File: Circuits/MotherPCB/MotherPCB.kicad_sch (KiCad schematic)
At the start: 1 part, among them U20 Teensy_4.1

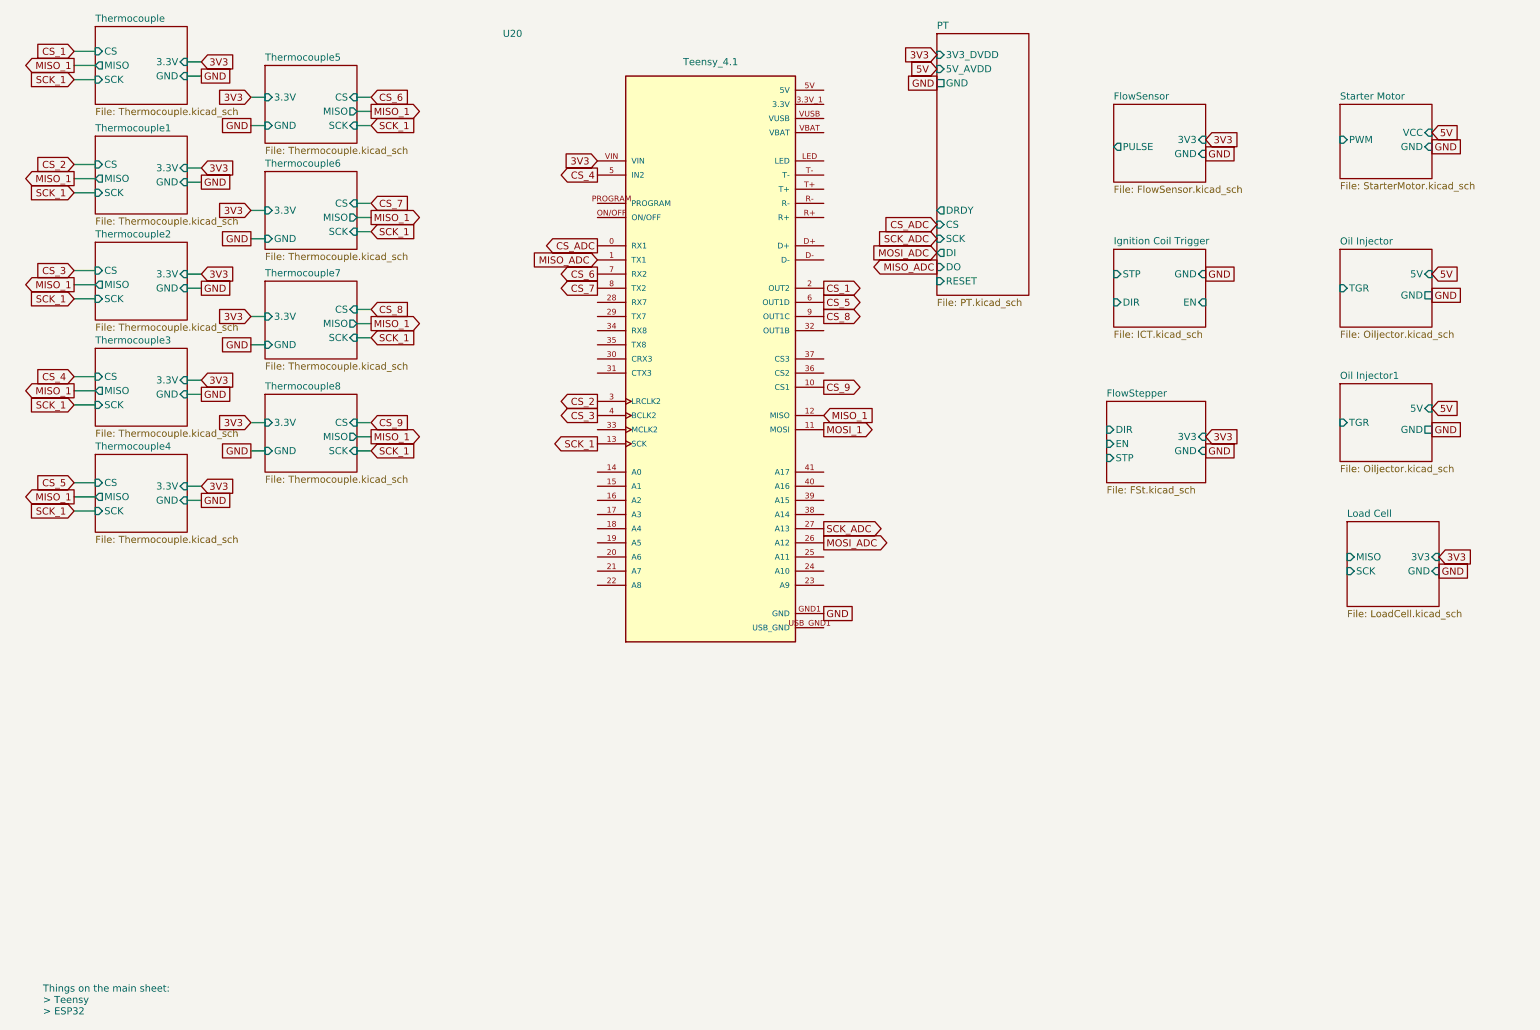
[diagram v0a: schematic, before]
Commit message: Schematic Finished
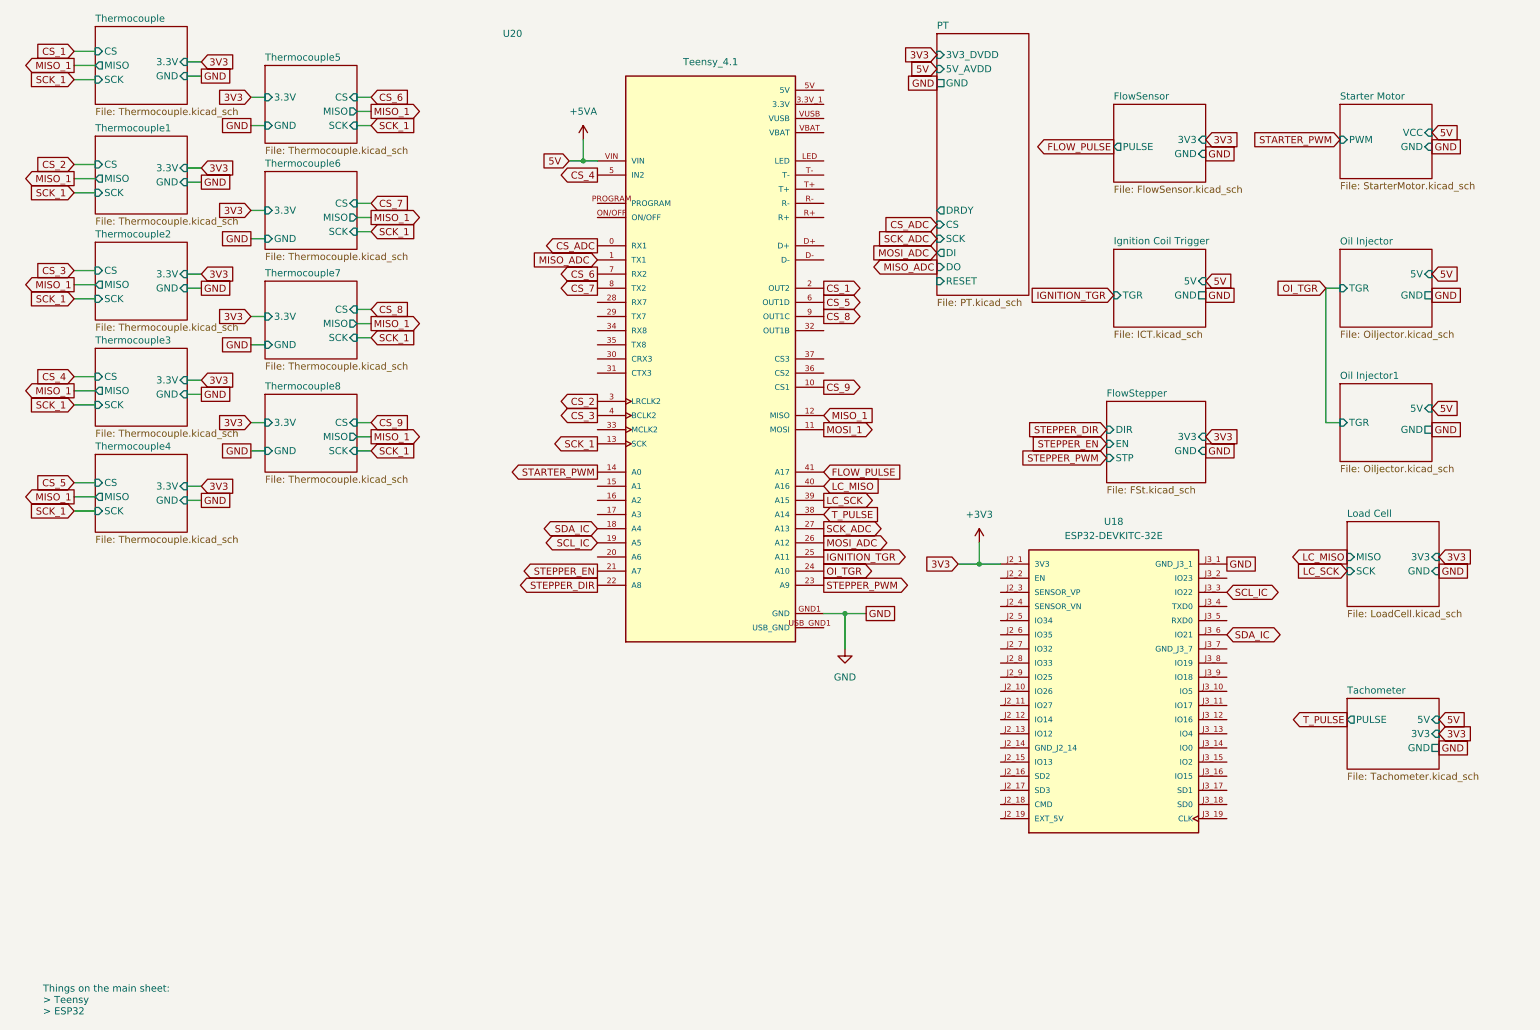
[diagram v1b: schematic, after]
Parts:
- added U18: ESP32-DEVKITC-32E, ESP32-DEVKITC-32E:MODULE_ESP32-DEVKITC-32E, symbol Additional_Components:ESP32-DEVKITC-32E
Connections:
- net GND: now also U18.J3_1 (GND_J3_1)
- net STARTER_PWM: now reaches U20.14 (A0)
- net SDA_IC: now reaches U20.18 (A4)
- net SDA_IC: now also U18.J3_6 (IO21)
- net SCL_IC: now reaches U20.19 (A5)
- net SCL_IC: now also U18.J3_3 (IO22)
- net STEPPER_EN: now reaches U20.21 (A7)
- net STEPPER_DIR: now reaches U20.22 (A8)
- net STEPPER_PWM: now reaches U20.23 (A9)
- net OI_TGR: now reaches U20.24 (A10)
- net IGNITION_TGR: now reaches U20.25 (A11)
- net T_PULSE: now reaches U20.38 (A14)
- net LC_SCK: now reaches U20.39 (A15)
- net LC_MISO: now reaches U20.40 (A16)
- net FLOW_PULSE: now reaches U20.41 (A17)
- net 3V3 renamed +5VA
- new net +3V3: U18.J2_1 (3V3)
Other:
- added sheet Tachometer (Tachometer.kicad_sch)
- sheet Ignition Coil Trigger ports: added 5V, TGR; removed DIR, EN, STP

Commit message: Fixed some broken footprints
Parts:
- U18: footprint ESP32-DEVKITC-32E:MODULE_ESP32-DEVKITC-32E -> Additional_Components:MODULE_ESP32-DEVKITC-32E
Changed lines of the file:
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@@
 			)
 		)
-		(property "Footprint" "ESP32-DEVKITC-32E:MODULE_ESP32-DEVKITC-32E"
+		(property "Footprint" "Additional_Components:MODULE_ESP32-DEVKITC-32E"
 			(at 210.82 135.89 0)
 			(effects
